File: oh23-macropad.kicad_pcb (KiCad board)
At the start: 2 copper layers, 1 part, among them U1 MOUDLE-SEEEDUINO-XIAO

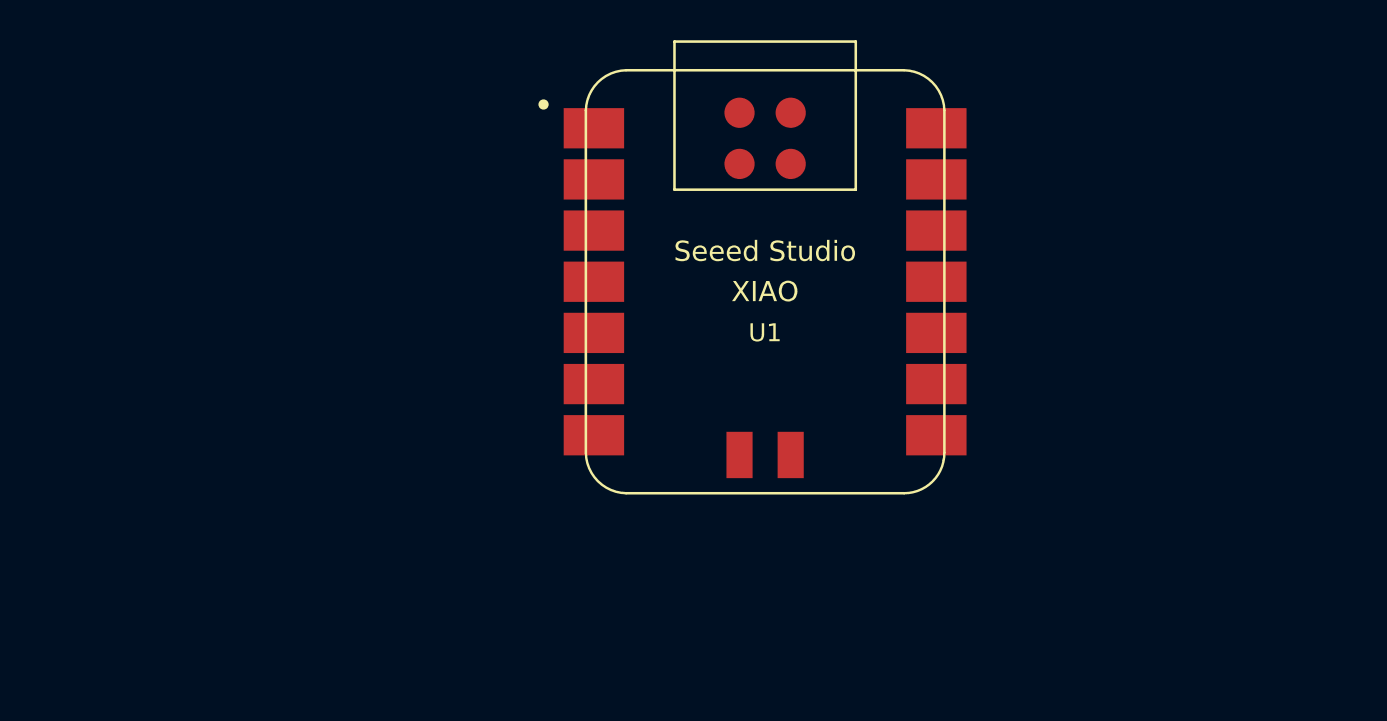
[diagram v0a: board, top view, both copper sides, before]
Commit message: Add design
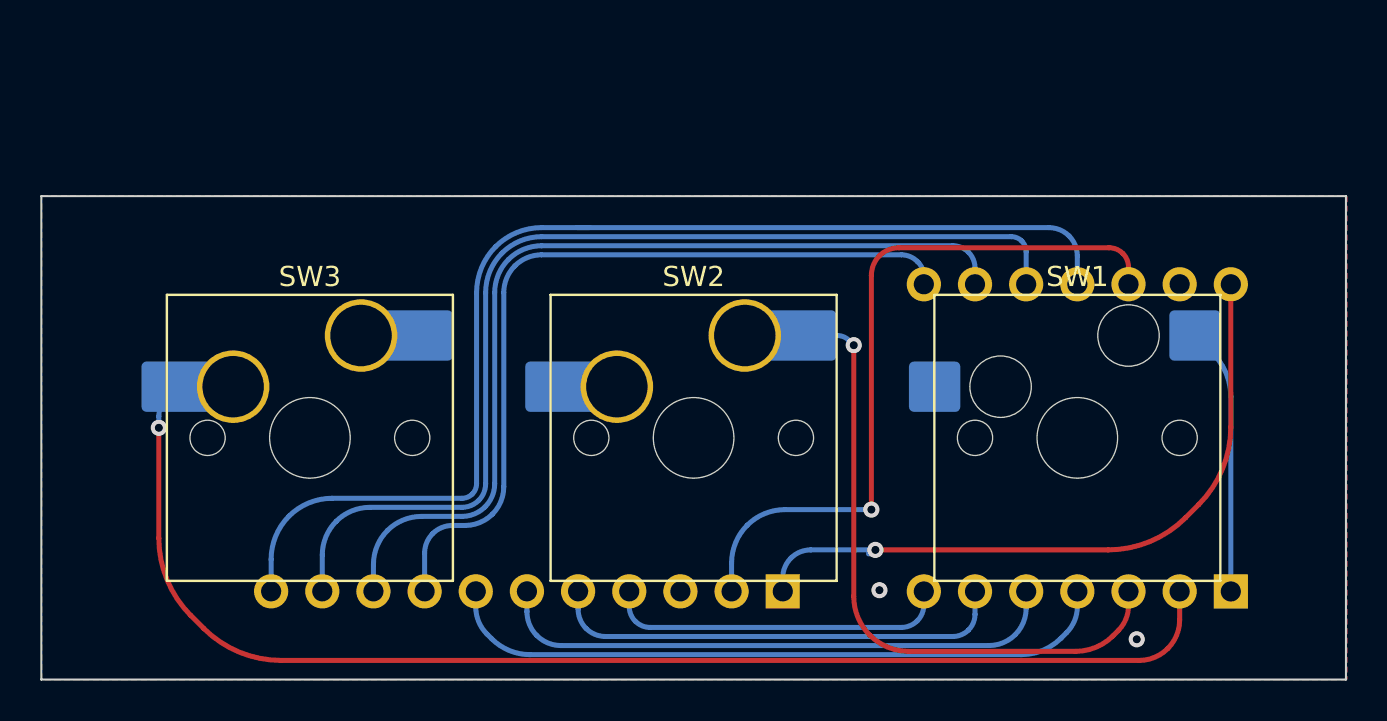
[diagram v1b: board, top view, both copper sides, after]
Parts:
- added J1: Conn_01x11, Connector_PinHeader_2.54mm:PinHeader_1x11_P2.54mm_Vertical, B.Cu at (103.4, 100.4)
- added SW1: SW_Push, Switch_Keyboard_Hotswap_Kailh:SW_Hotswap_Kailh_MX_1.00u, F.Cu at (118.0, 92.8)
- added SW2: SW_Push, Switch_Keyboard_Hotswap_Kailh:SW_Hotswap_Kailh_MX_plated_1.00u, F.Cu at (99.0, 92.8)
- added SW3: SW_Push, Switch_Keyboard_Hotswap_Kailh:SW_Hotswap_Kailh_MX_plated_1.00u, F.Cu at (79.9, 92.8)
- U1: footprint Seeed Studio XIAO Series Library:XIAO-SAMD21-RP2040-14P-2.54-21X17.8MM (Seeeduino XIAO) -> Seeed Studio XIAO Series Library:XIAO-Generic-Thruhole-14P-2.54-21X17.8MM; moved to B.Cu
- moved U1 17.3 mm to (118.0, 92.8), turned to 90 degrees
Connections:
- U1 pad 1: unconnected-(U1-Pad1) -> Net-(U1-Pad1)
- U1 pad 10: unconnected-(U1-Pad10) -> /GP04_D09
- U1 pad 11: unconnected-(U1-Pad11) -> /GP03_D10
- U1 pad 12: unconnected-(U1-Pad12) -> +3V3
- U1 pad 13: unconnected-(U1-Pad13) -> GND
- U1 pad 14: unconnected-(U1-Pad14) -> +5V
- U1 pad 2: unconnected-(U1-Pad2) -> Net-(U1-Pad2)
- U1 pad 3: unconnected-(U1-Pad3) -> Net-(U1-Pad3)
- U1 pad 4: unconnected-(U1-Pad4) -> /GP29_D03
- U1 pad 5: unconnected-(U1-Pad5) -> /GP06_D04
- U1 pad 6: unconnected-(U1-Pad6) -> /GP07_D05
- U1 pad 7: unconnected-(U1-Pad7) -> /GP00_D06
- U1 pad 8: unconnected-(U1-Pad8) -> /GP01_D07
- U1 pad 9: unconnected-(U1-Pad9) -> /GP02_D08
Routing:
- net Net-(U1-Pad2): track 0.00 -> 64.4 mm, vias 0 -> 1
- net /GP03_D10: track 0.00 -> 57.8 mm
- net /GP04_D09: track 0.00 -> 51.8 mm
- net /GP02_D08: track 0.00 -> 45.7 mm
- net /GP01_D07: track 0.00 -> 40.2 mm
- net +3V3: track 0.00 -> 36.4 mm, vias 0 -> 1
- net +5V: track 0.00 -> 34.5 mm, vias 0 -> 1
- net /GP29_D03: track 0.00 -> 33.8 mm
- net Net-(U1-Pad3): track 0.00 -> 32.3 mm, vias 0 -> 1
- net /GP06_D04: track 0.00 -> 28.6 mm
- net /GP07_D05: track 0.00 -> 23.1 mm
- net /GP00_D06: track 0.00 -> 17.3 mm
- net Net-(U1-Pad1): track 0.00 -> 13.3 mm
- net GND: vias 0 -> 2
- added copper zone on B.Cu, net GND
- added copper zone on F.Cu, net GND
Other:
- board outline added: 64.8 x 24 mm
- board text added: "3-key Macropad"
- board text added: "3V3"
- board text added: "5V"
- board text added: "GND"
- board text added: "GP0"
- board text added: "GP1"
- board text added: "GP2"
- board text added: "GP29"
- board text added: "GP3"
- board text added: "GP4"
- board text added: "GP6"
- board text added: "GP7"
- board text added: "I2C1"
- board text added: "SPI0"
